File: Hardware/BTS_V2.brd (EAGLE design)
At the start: 113 x 79.4 mm, 64 parts, among them IC1 TPA3140D2PWP, IC2 BLK-MD-SPK-B, J1 SPKR_OUT, J2 RN52BoB_R, J3 RN52BoB_L, J4 TFT_CONNECTION, J6 HC-05, T3_2 TEENSY_3.1-3.2_DIL

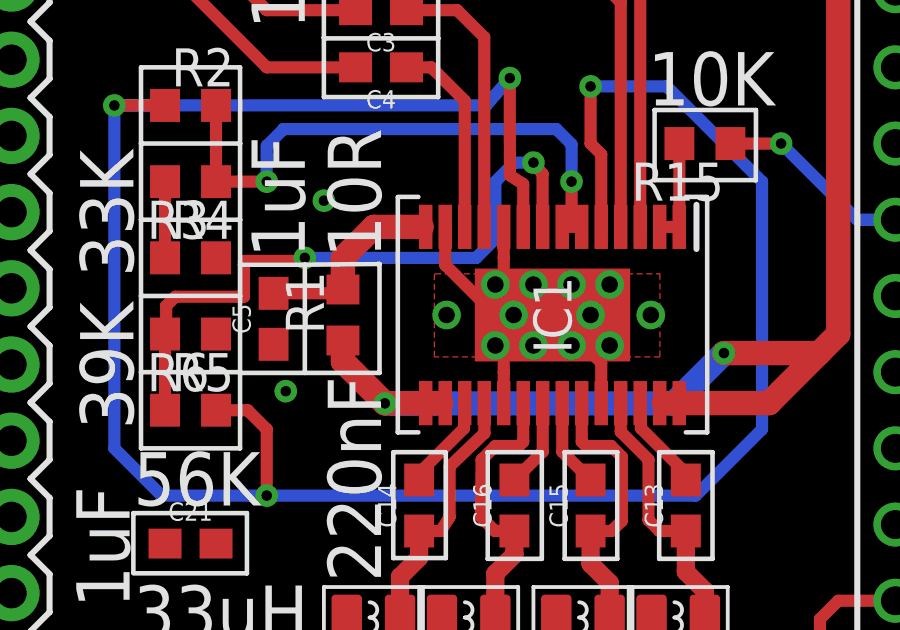
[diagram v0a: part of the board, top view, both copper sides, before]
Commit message: Still working on figuring out an error w/ the board
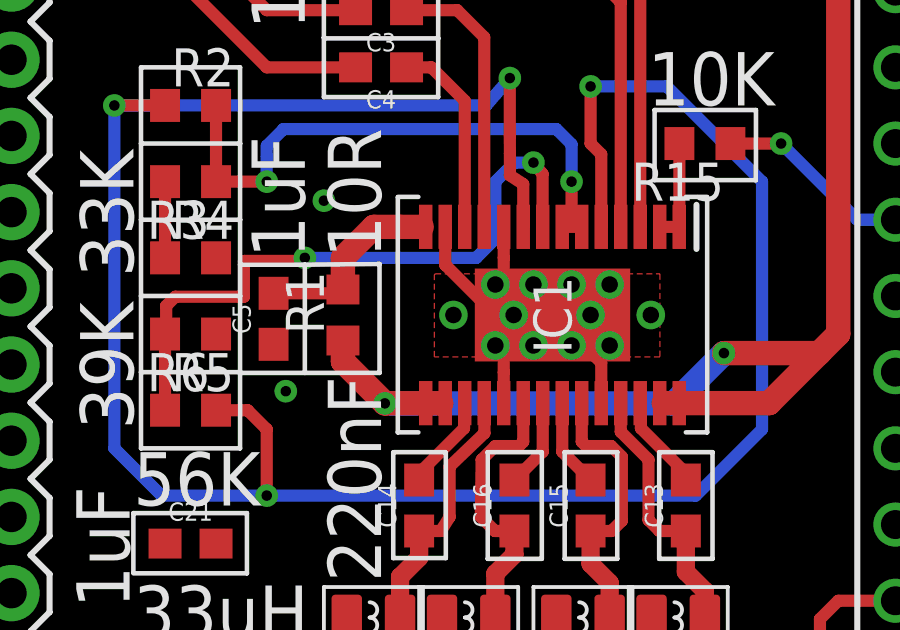
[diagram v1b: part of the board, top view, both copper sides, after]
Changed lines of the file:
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@@
 <wire x1="33.64" y1="29.03" x2="47.64" y2="29.03" width="0.4064" layer="1"/>
 <via x="71.755" y="28.956" extent="1-16" drill="0.55"/>
-<via x="70.1294" y="27.94" extent="1-16" drill="0.55"/>
+<via x="70.358" y="27.94" extent="1-16" drill="0.55"/>
 <via x="71.755" y="26.924" extent="1-16" drill="0.55"/>
 <via x="73.025" y="26.924" extent="1-16" drill="0.55"/>
